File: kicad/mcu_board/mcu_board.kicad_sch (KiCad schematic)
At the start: 36 parts, among them J1 Button 1, J2 Humidity, J3 IR, J5 AVR Programmer, SW1 RST_Btn, U1 LM2575D2T-3.3R4G, U2 VOM617A, U3 LM2575D2T-5R4G, U4 ATmega328-A, Y1 16MHz

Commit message: MCU board WIP
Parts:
- removed J?: Conn_01x01_Male, symbol Connector:Conn_01x01_Male
- removed R?: R_Small, symbol Device:R_Small
- removed U?: LTC4151xMS, Package_SO:MSOP-10_3x3mm_P0.5mm, symbol Analog_ADC:LTC4151xMS
- added IC?: LTC4151IMS-1#PBF, SOP50P490X110-10N, symbol SamacSys_Parts:LTC4151IMS-1#PBF
- added J4: Solar Panel, symbol Connector:Conn_01x02_Male
- added Q? (x2): MOCD207M, SOIC127P594X363-8N, symbol SamacSys_Parts:MOCD207M
- added R? (x2): 10k, symbol Device:R
- added R? (x2): 20k, symbol Device:R
- added R? (x2): 0.51k, symbol Device:R
- added R?: 5.1k, symbol Device:R
- added R?: ERJ-3BWFR020V, ERJ3_B_BQ_BW_LW_(0603), symbol SamacSys_Parts:ERJ-3BWFR020V
- added U?: ATmega328-P, Package_DIP:DIP-28_W7.62mm, symbol MCU_Microchip_ATmega:ATmega328-P
- R6: value 10k -> R_Small
- SW1: value RST_Btn -> RST Button
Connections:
- net +24V: now also IC?.1 (SENSE+), IC?.2 (VIN), IC?.3 (ADR1), R?.1
- net +3V3: now also R?.2, R?.2, R?.2, R?.2
- net GND: now also Q?.7 (EMITTER_1); no longer J1.2 (Pin_2)
- new net: Q?.4 (CATHODE_2), Q?.8 (COLLECTOR_1), R?.1
- new net: IC?.7 (SDAI), Q?.6 (COLLECTOR_2), R?.1
- new net: IC?.6 (SCL), Q?.8 (COLLECTOR_1), R?.1
- new net: IC?.8 (~{SDAO}), Q?.1 (ANODE_1), R?.1
- new net: Q?.1 (ANODE_1), R?.1
- new net: Q?.3 (ANODE_2), R?.1
- new net: Q?.2 (CATHODE_1), R?.1
- new net: U?.22 (GND), U?.8 (GND)
- new net 24_OUT: IC?.10 (SENSE-), R?.2, R?.2, R?.2, R?.2
- new net GNDPWR: IC?.4 (ADR0), IC?.5 (ADIN), IC?.9 (GND), J1.2 (Pin_2), Q?.2 (CATHODE_1), Q?.5 (EMITTER_2), Q?.7 (EMITTER_1)
- no-connect marks 1 -> 0
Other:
- moved on the sheet: D3, J1, J2, J3, R1, R2, R3, R4, R5, U2, U4

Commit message: MCU board WIP
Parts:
- removed C1, C3: 100uF, Capacitor_THT:C_Radial_D8.0mm_H11.5mm_P3.50mm, symbol Device:C_Polarized_Small
- removed C2, C5: 330uF, Capacitor_THT:CP_Radial_D8.0mm_P3.50mm, symbol Device:C_Polarized_Small
- removed D1, D2: VS-30WQ04FNTR-M3, Package_TO_SOT_SMD:TO-252-2, symbol Device:D_Schottky
- removed D3: LED, symbol Device:LED
- removed IC?: LTC4151IMS-1#PBF, SOP50P490X110-10N, symbol SamacSys_Parts:LTC4151IMS-1#PBF
- removed J5: AVR Programmer, symbol Connector_Generic:Conn_02x03_Odd_Even
- removed L1, L2: 330uH, Inductor_THT:L_Toroid_Vertical_L31.8mm_W15.9mm_P13.50mm_Bourns_5700, symbol Device:L_Small
- removed Q? (x2): MOCD207M, SOIC127P594X363-8N, symbol SamacSys_Parts:MOCD207M
- removed R2, R3, R4, R5: R_Small, symbol Device:R_Small
- removed R? (x2): 10k, symbol Device:R
- removed R? (x2): 20k, symbol Device:R
- removed R? (x2): 0.51k, symbol Device:R
- removed R?: 5.1k, symbol Device:R
- removed R?: ERJ-3BWFR020V, ERJ3_B_BQ_BW_LW_(0603), symbol SamacSys_Parts:ERJ-3BWFR020V
- removed U1: LM2575D2T-3.3R4G, Package_TO_SOT_SMD:TO-263-5_TabPin3, symbol Regulator_Switching:LM2575-3.3BU
- removed U2: VOM617A, Package_DIP:DIP-4_W7.62mm, symbol Isolator:SFH617A-1
- removed U3: LM2575D2T-5R4G, Package_TO_SOT_SMD:TO-263-5_TabPin3, symbol Regulator_Switching:LM2575-5.0BU
- removed U4: ATmega328-A, Package_QFP:TQFP-32_7x7mm_P0.8mm, symbol MCU_Microchip_ATmega:ATmega328-A
- added C1: 0.1uF, symbol Device:C_Small
- added C?: 100uF, symbol Device:C_Small
- added H1, H2, H3, H4: MountingHole, symbol Mechanical:MountingHole
- added J10: Lights, symbol Connector:Conn_01x04_Male
- added J5: Photoresistor, symbol Connector:Conn_01x02_Male
- added J6: 24V In, symbol Connector:Conn_01x02_Male
- added J7: 5V Out, symbol Connector:Conn_01x03_Male
- added J8: Programmer, symbol Connector:AVR-ISP-6
- added J9: Power Board, symbol Connector:Conn_01x03_Male
- added PS5: TMR_2-2411WIN, TMR-2_SERIES, symbol SamacSys_Parts:TMR_2-2411WIN
- C11: value C_Small -> 10uF
- J1: value Button 1 -> Buttons
- J4: value Solar Panel -> Power Monitor
- R1, R6: value R_Small -> 10k
- gave numbers to parts that had none: 1
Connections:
- net GNDPWR is gone; now on net Bike: J1.2 (Pin_2)
- net SCL_DHT is gone; now on net GND1: J2.3 (Pin_3)
- net SDA_DHT is gone; now on net SDA: J2.2 (Pin_2)
- net +24V: now also J6.1 (Pin_1), PS5.2 (+VIN_(VCC)); no longer R1.2
- net +5V: now also U1.20 (AVCC), U1.7 (VCC), C?.1, J5.1 (Pin_1), J7.1 (Pin_1), J8.2 (VCC), PS5.6 (+VOUT)
- net GND: now also J6.2 (Pin_2), PS5.1 (-VIN_(GND)); no longer C10.2, C11.2, C12.2, C4.2, C6.2, C7.2, C8.2, C9.2, J2.4 (Pin_4), J3.3 (Pin_3), SW1.3 (B), SW1.4 (B)
- net MCU_MISO: now also U1.18 (PB4), J8.1 (MISO)
- net MCU_MOSI: now also U1.17 (PB3), J8.4 (MOSI)
- net MCU_N_RESET: now also U1.1 (~{RESET}/PC6), J8.5 (~{RST})
- net MCU_SCK: now also U1.19 (PB5), J8.3 (SCK)
- net MCU_XTAL1: now also U1.9 (XTAL1/PB6)
- net MCU_XTAL2: now also U1.10 (XTAL2/PB7)
- net Vo: now also U1.24 (PC1)
- net Pedestrian: now reaches J1.1 (Pin_1)
- net Pedestrian: now also U1.13 (PD7)
- net SCL: now reaches J4.1 (Pin_1)
- net SCL: now also J2.4 (Pin_4), U1.28 (PC5)
- net SDA: now reaches J4.2 (Pin_2)
- net SDA: now also U1.27 (PC4)
- net Photoresistor: now reaches R1.1
- net Photoresistor: now also U1.23 (PC0), J5.2 (Pin_2)
- net Red: now reaches U1.11 (PD5)
- net Red: now also J10.1 (Pin_1)
- net Green: now reaches U1.12 (PD6)
- net Green: now also J10.2 (Pin_2)
- net Bike: now reaches U1.14 (PB0)
- net Yellow: now reaches U1.15 (PB1)
- net Yellow: now also J10.3 (Pin_3)
- net Walk_Light: now reaches U1.16 (PB2)
- net Walk_Light: now also J10.4 (Pin_4)
- net at U1.21 (AREF): now also C1.1
- net GND1: now reaches U1.22 (GND), U1.8 (GND)
- net GND1: now also C10.2, C11.2, C12.2, C4.2, C6.2, C7.2, C8.2, C9.2, J3.3 (Pin_3), R1.2, SW1.3 (B), SW1.4 (B), C1.2, C?.2, J7.2 (Pin_2), J7.3 (Pin_3), J8.6 (GND), PS5.7 (-VOUT)
- net Solar: now reaches U1.4 (PD2)
- net Solar: now also J9.1 (Pin_1)
- net Grid: now reaches U1.5 (PD3)
- net Grid: now also J9.2 (Pin_2)
- net Resistor: now reaches U1.6 (PD4)
- net Resistor: now also J9.3 (Pin_3)
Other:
- note added: "24V to 5V Converter"
- note added: "Crystal Oscillator"
- note added: "ISP"
- note added: "Mounting Holes"
- note added: "Outputs to Power and Light Boards"
- note added: "Reset Button"
- note added: "Sensor Inputs"
- note removed: "24V to 3.3V Buck"
- note removed: "24V to 5V Buck"
- note removed: "Bike/pedestrian buttons"
- moved on the sheet: C10, C11, C12, C4, C6, C7, C8, C9, J2, J3, R6, SW1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

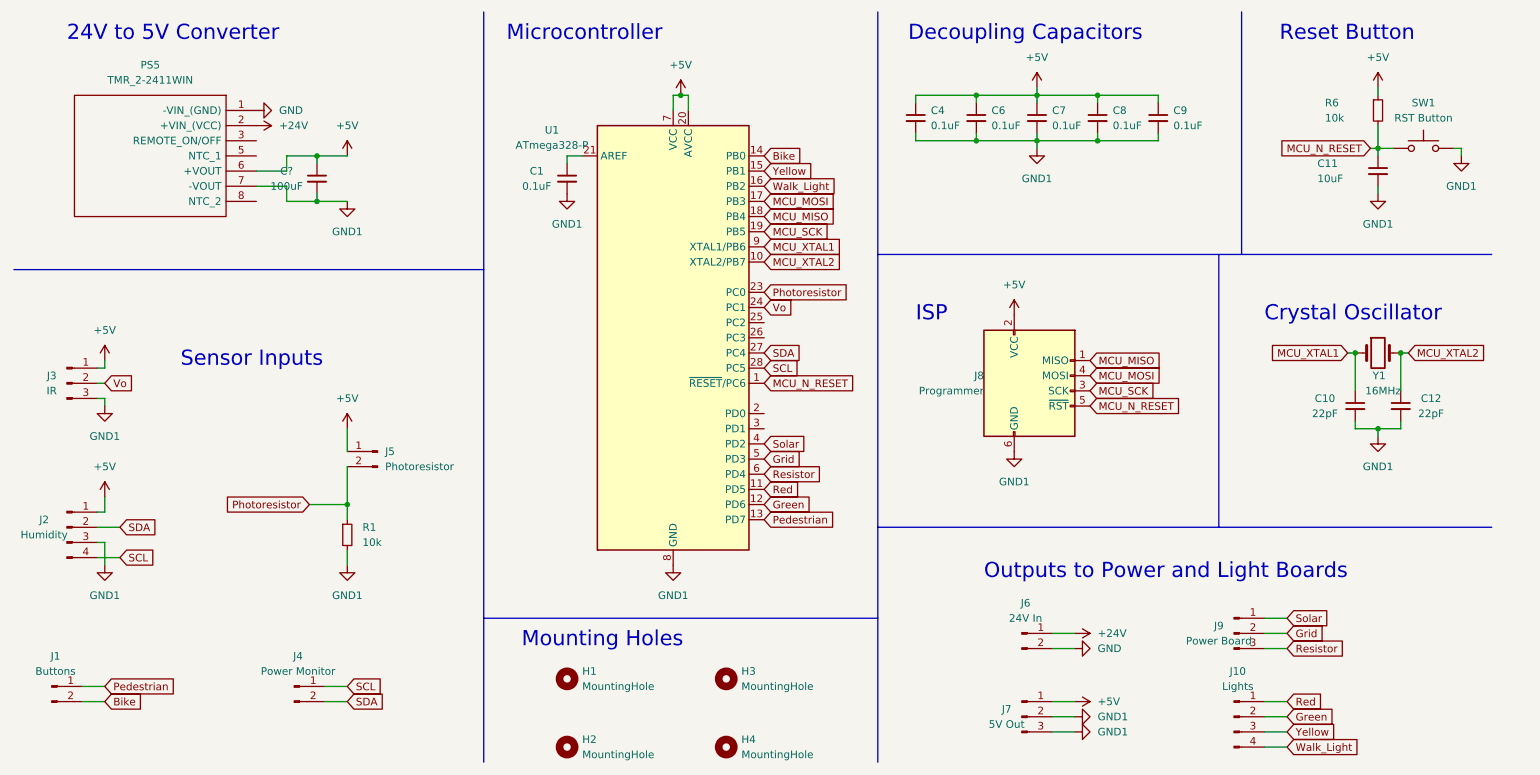
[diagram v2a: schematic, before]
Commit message: working on MCU
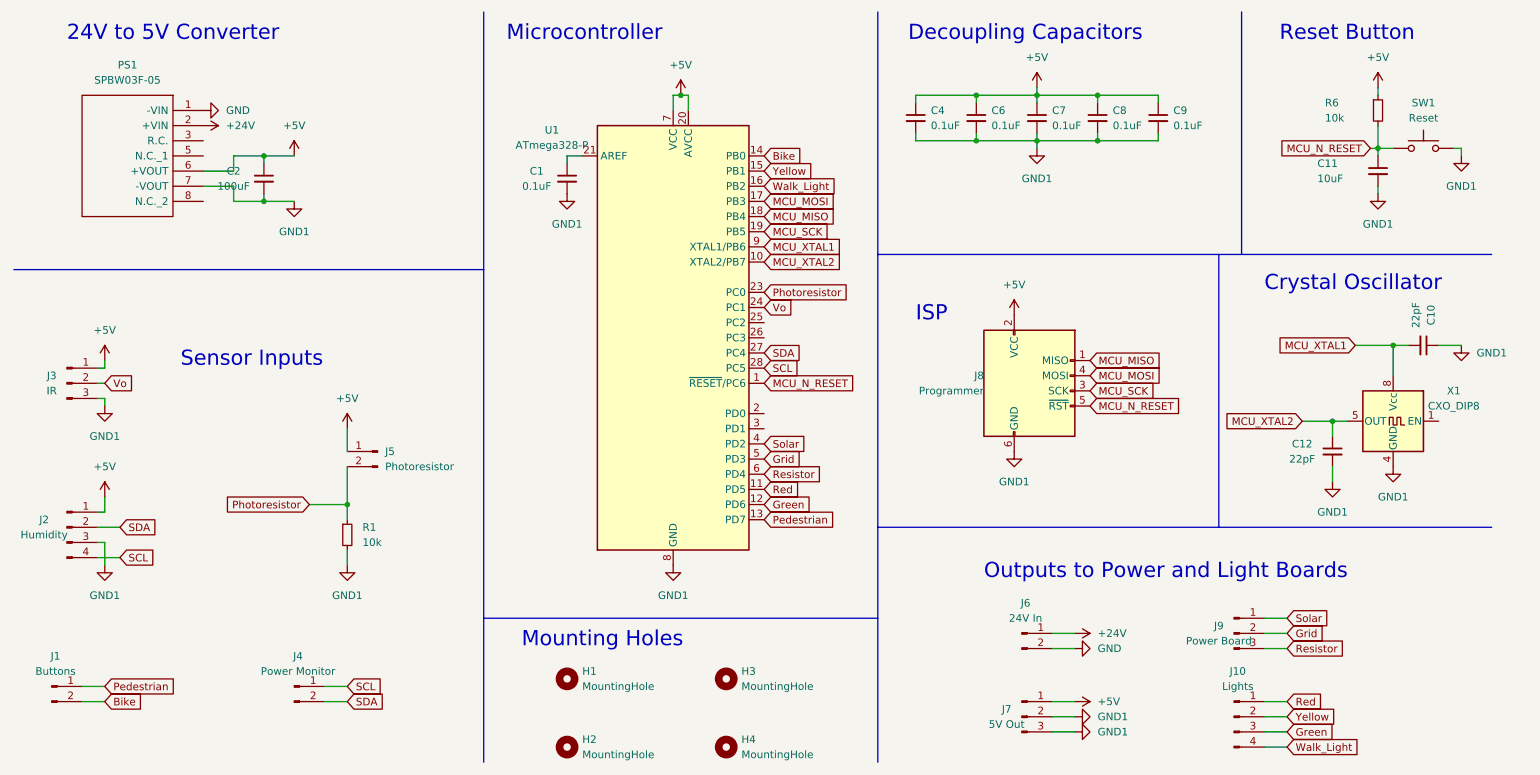
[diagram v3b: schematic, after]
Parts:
- removed PS5: TMR_2-2411WIN, TMR-2_SERIES, symbol SamacSys_Parts:TMR_2-2411WIN
- removed SW1: RST Button, symbol Switch:SW_MEC_5G
- removed Y1: 16MHz, symbol Device:Crystal
- added PS1: SPBW03F-05, SamacSys_Parts:SPBW06F05, symbol SamacSys_Parts:SPBW03F-05
- added SW1: Reset, Button_Switch_SMD:SW_SPST_TL3305B, symbol Switch:SW_Push
- added X1: CXO_DIP8, Oscillator:Oscillator_DIP-8, symbol Oscillator:CXO_DIP8
- C1, C4, C6, C7, C8, C9: footprint (none) -> Capacitor_SMD:C_0201_0603Metric_Pad0.64x0.40mm_HandSolder
- C10, C11, C12: footprint (none) -> Capacitor_SMD:C_0603_1608Metric_Pad1.08x0.95mm_HandSolder
- C2: renamed from C?; footprint (none) -> Capacitor_SMD:C_1206_3216Metric_Pad1.33x1.80mm_HandSolder
- H1, H2, H3, H4: footprint (none) -> MountingHole:MountingHole_3.2mm_M3
- J1, J4, J5, J6: footprint (none) -> Connector_PinHeader_2.54mm:PinHeader_1x02_P2.54mm_Vertical
- J10, J2: footprint (none) -> Connector_PinHeader_2.54mm:PinHeader_1x04_P2.54mm_Vertical
- J3, J7, J9: footprint (none) -> Connector_PinHeader_2.54mm:PinHeader_1x03_P2.54mm_Vertical
- J8: footprint (none) -> Connector_IDC:IDC-Header_2x03_P2.54mm_Vertical
- R1, R6: footprint (none) -> Resistor_SMD:R_0805_2012Metric_Pad1.20x1.40mm_HandSolder
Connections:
- net +24V: now also PS1.2 (+VIN)
- net +5V: now also PS1.6 (+VOUT)
- net GND: now also PS1.1 (-VIN)
- net GND1: now also C10.1, PS1.7 (-VOUT), SW1.2, X1.4 (GND); no longer C10.2
- net Green: now also J10.3 (Pin_3); no longer J10.2 (Pin_2)
- net MCU_N_RESET: now also SW1.1
- net MCU_XTAL1: now also C10.2, X1.8 (Vcc); no longer C10.1
- net MCU_XTAL2: now also X1.5 (OUT)
- net Yellow: now also J10.2 (Pin_2); no longer J10.3 (Pin_3)
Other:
- moved on the sheet: C10, C12, C2

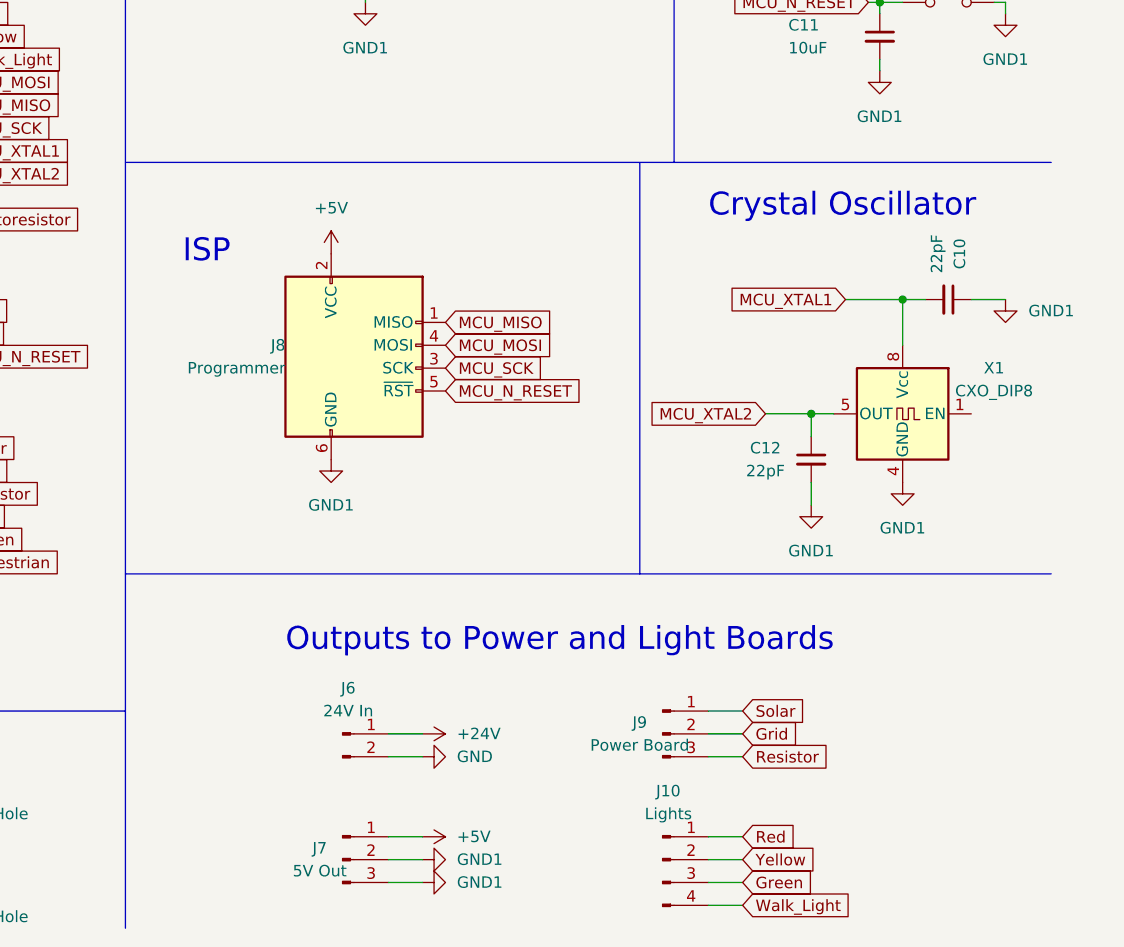
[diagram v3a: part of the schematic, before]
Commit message: finished up MCU board
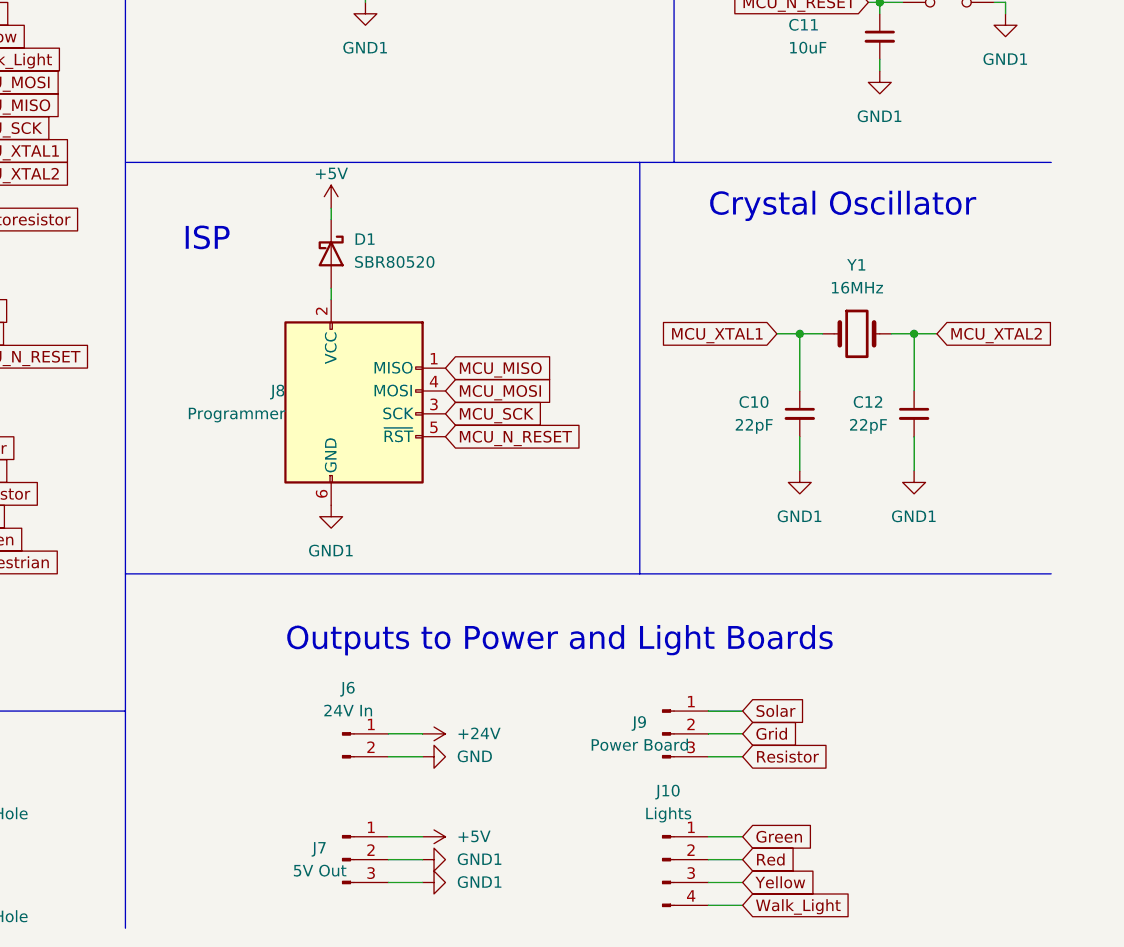
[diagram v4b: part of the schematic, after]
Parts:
- removed X1: CXO_DIP8, Oscillator:Oscillator_DIP-8, symbol Oscillator:CXO_DIP8
- added D1: SBR80520, Diode_SMD:D_SOD-123, symbol Device:D_Schottky
- added Y1: 16MHz, Crystal:Crystal_HC49-U_Vertical, symbol Device:Crystal
- C1, C4, C6, C7, C8, C9: footprint Capacitor_SMD:C_0201_0603Metric_Pad0.64x0.40mm_HandSolder -> Capacitor_SMD:C_0603_1608Metric_Pad1.08x0.95mm_HandSolder
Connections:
- net +5V: now also D1.1 (K); no longer J8.2 (VCC)
- net GND1: now also C10.2; no longer C10.1
- net Green: now also J10.1 (Pin_1); no longer J10.3 (Pin_3)
- net MCU_XTAL1: now also C10.1, Y1.1; no longer C10.2
- net MCU_XTAL2: now also Y1.2
- net Red: now also J10.2 (Pin_2); no longer J10.1 (Pin_1)
- net Yellow: now also J10.3 (Pin_3); no longer J10.2 (Pin_2)
- new net: D1.2 (A), J8.2 (VCC)
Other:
- moved on the sheet: C10, C12, J8
